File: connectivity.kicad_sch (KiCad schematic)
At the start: 28 parts, among them J10 Screw_Terminal_01x05, J11 RJ45_Hanrun_HR911105A_Horizon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, J8 Conn_02x01, J9 Conn_02x01, U6 TJA1042T-3, U7 LAN8742A, Y3 25 MHz

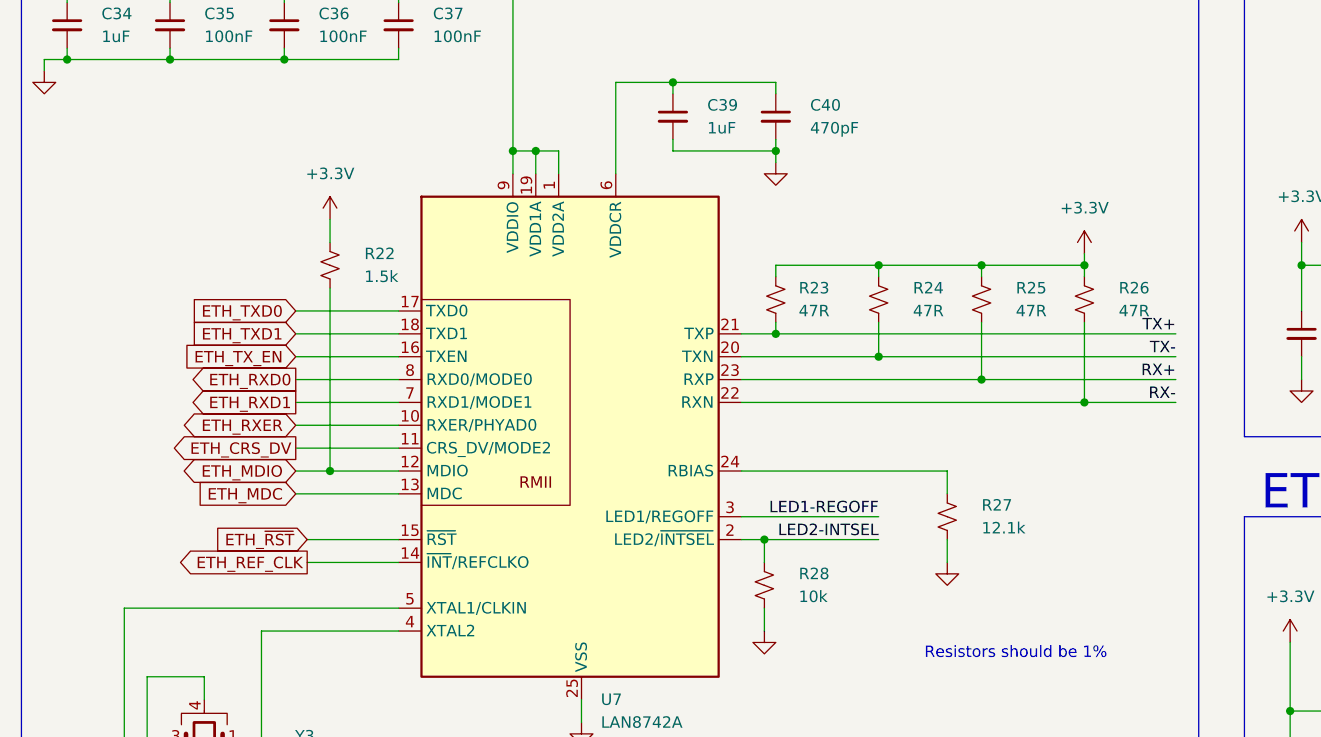
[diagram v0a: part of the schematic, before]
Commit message: Timeline is not real
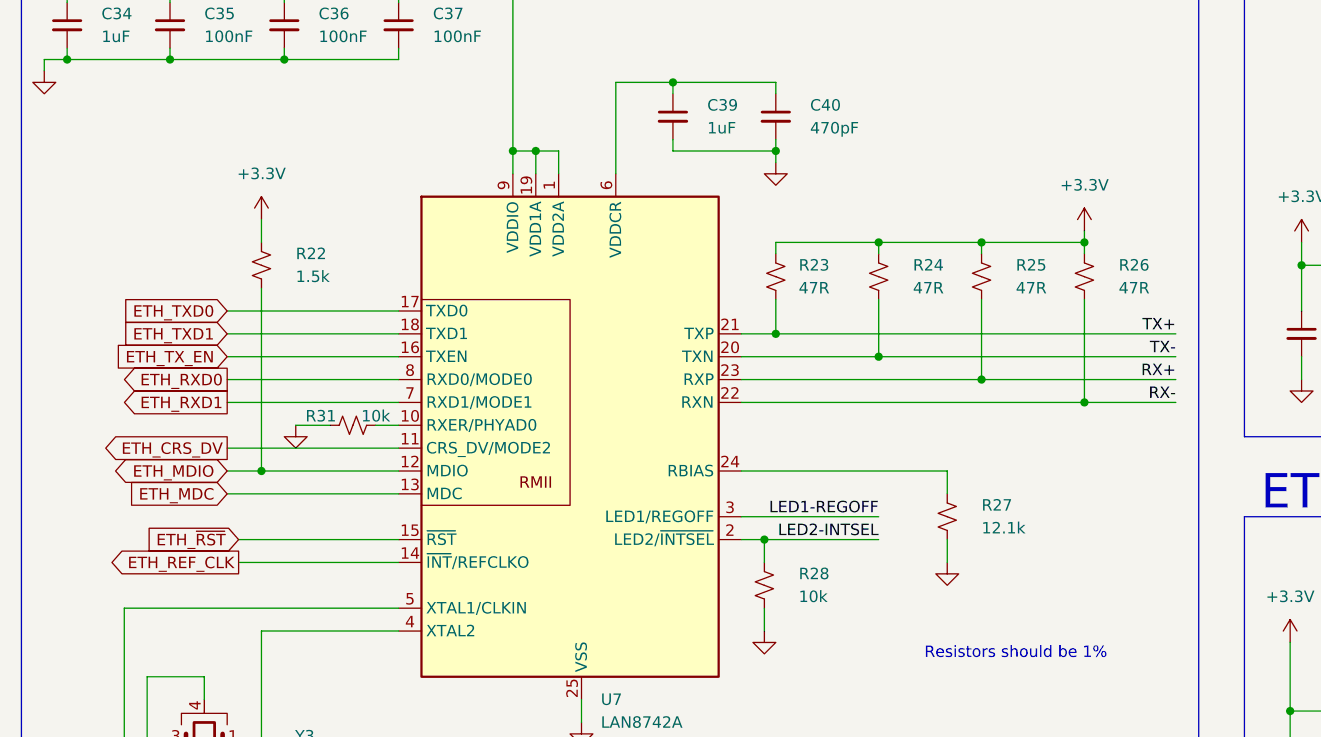
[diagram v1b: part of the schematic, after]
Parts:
- added R31: 10k, APRLPrints:R_0603, symbol Device:R_Small_US
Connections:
- net GND: now also R31.1
- net ETH_RXER: no longer names the net of U7.10 (RXER/PHYAD0)
- net ETH_RXER: now also R31.2
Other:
- moved on the sheet: R22, R23, R24, R25, R26
